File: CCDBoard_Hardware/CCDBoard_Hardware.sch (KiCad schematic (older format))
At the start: 19 parts

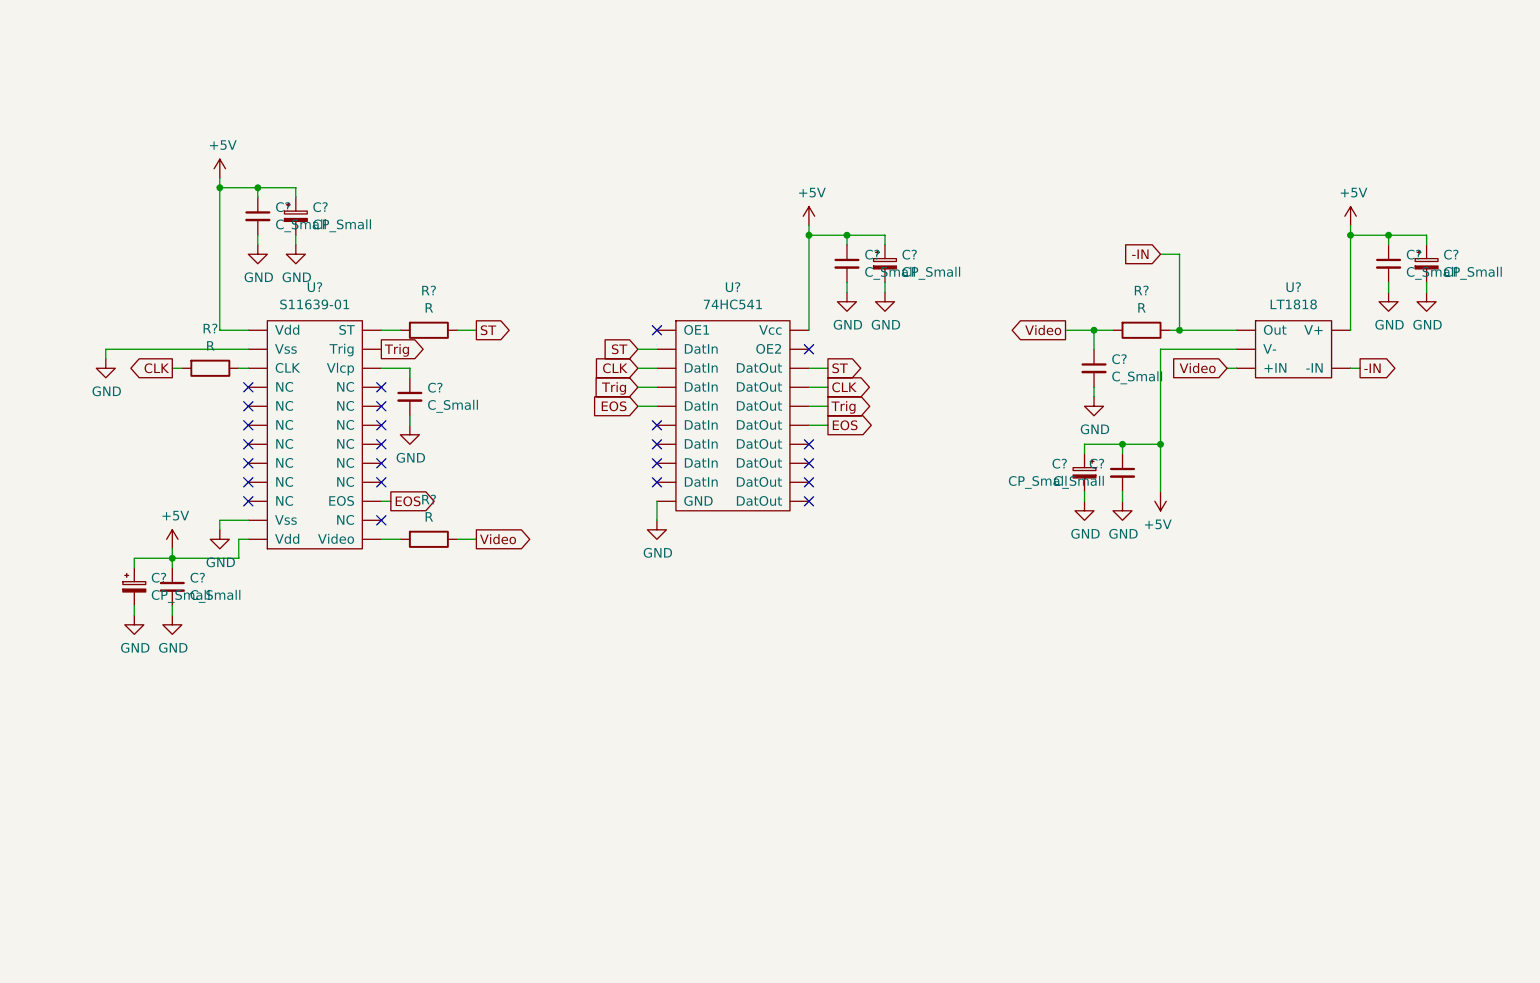
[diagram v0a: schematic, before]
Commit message: Further Edits
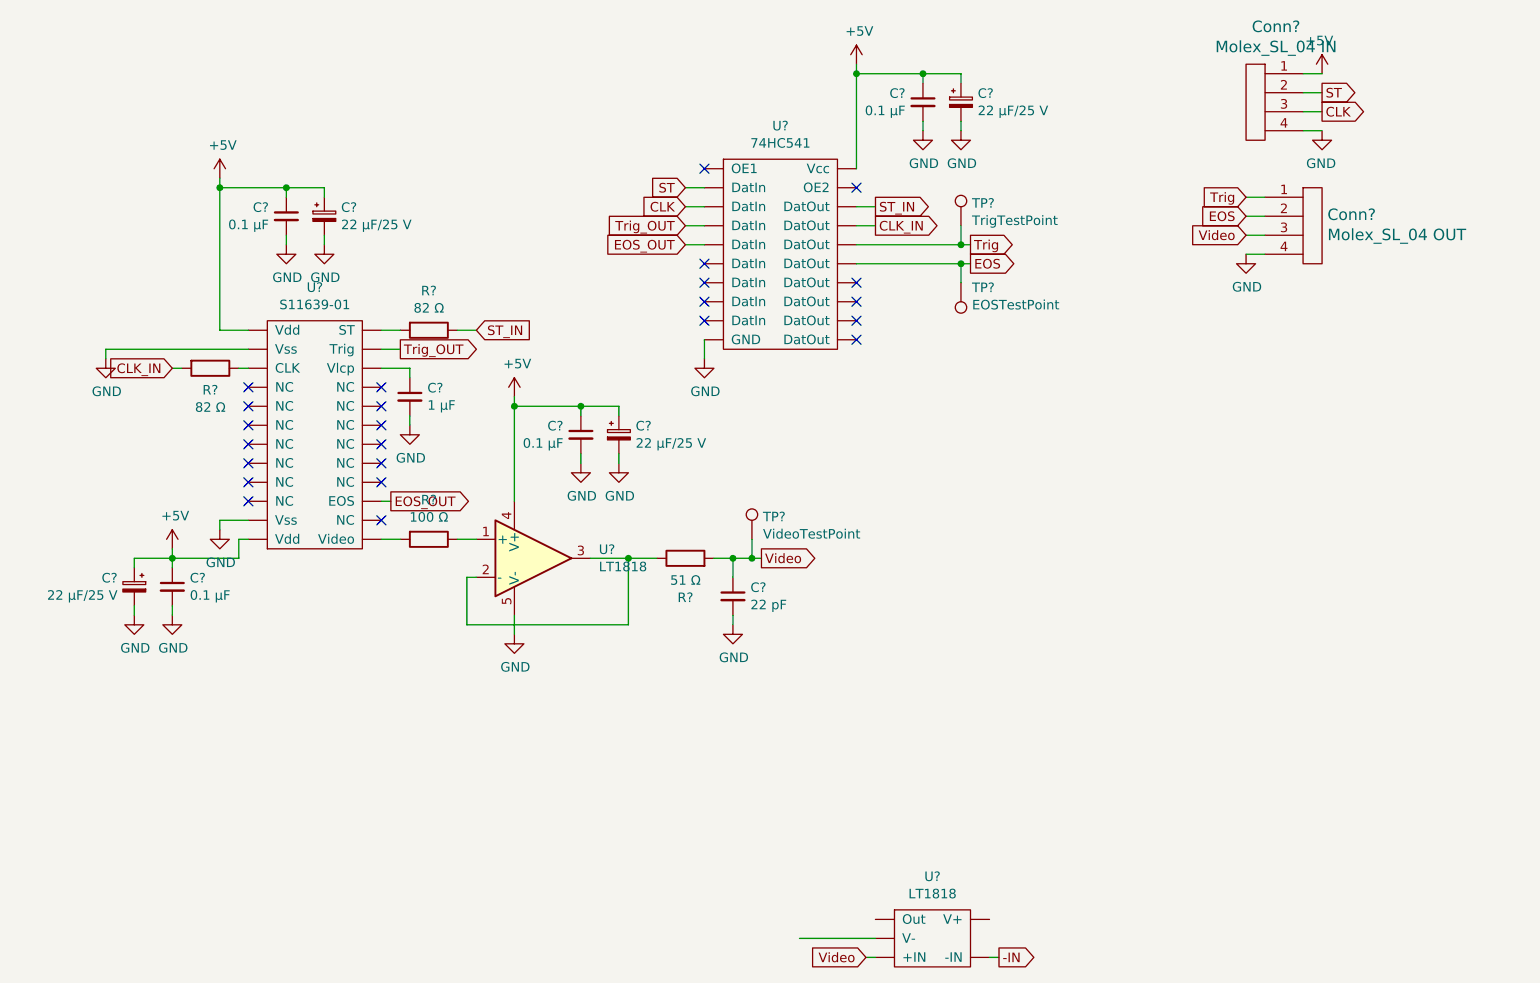
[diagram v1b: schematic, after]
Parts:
- removed C? (x3): C_Small, symbol Device:C_Small
- removed C? (x3): CP_Small, symbol Device:CP_Small
- added C? (x2): 0.1 µF, symbol Device:C_Small
- added C? (x2): 22 µF/25 V, symbol Device:CP_Small
- added Conn?: Molex_SL_04 IN, symbol MRDT_Connectors:Molex_SL_04
- added Conn?: Molex_SL_04 OUT, symbol MRDT_Connectors:Molex_SL_04
- added TP?: VideoTestPoint, symbol Connector:TestPoint
- added TP?: TrigTestPoint, symbol Connector:TestPoint
- added TP?: EOSTestPoint, symbol Connector:TestPoint
- added U?: LT1818, symbol pspice:OPAMP
- C? (x2): value C_Small -> 0.1 µF
- C? (x2): value CP_Small -> 22 µF/25 V
- C?: value C_Small -> 1 µF
- C?: value C_Small -> 22 pF
- R? (x2): value R -> 82 Ω
- R?: value R -> 100 Ω
- R?: value R -> 51 Ω
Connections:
- net +5V: now also C?.1, C?.1, C?.1, C?.1, Conn?.1, U?.4 (V+); no longer U?.~ (V-)
- net -IN: no longer R?.1
- net CLK: now also Conn?.3; no longer R?.2
- net EOS: now also Conn?.2, TP?.1; no longer U?.~ (Vss)
- net GND: now also C?.2, C?.2, C?.2, C?.2, Conn?.4, Conn?.4, U?.5 (V-)
- net ST: now also Conn?.2; no longer R?.1
- net Trig: now also Conn?.1, TP?.1; no longer U?.~ (Vss)
- net Video: now also Conn?.3, TP?.1; no longer R?.1
- net Trig_OUT: now reaches U?.~ (Vss)
- net Trig_OUT: now also U?.~ (Vcc)
- new net: R?.1, U?.1 (+)
- new net: R?.1, U?.2 (-), U?.3
- new net CLK_IN: R?.2, U?.~ (Vcc)
- new net EOS_OUT: U?.~ (Vcc), U?.~ (Vss)
- new net ST_IN: R?.1, U?.~ (Vcc)
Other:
- moved on the sheet: C?, R?, U?
